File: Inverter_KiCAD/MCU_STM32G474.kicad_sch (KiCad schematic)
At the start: 27 parts, among them J2 Conn_ST_STDC14, SW1 SW_Push, SW2 SW_Push, SW3 SW_Push, SW4 SW_Push, U18 STM32G474RETx, Y1 16M

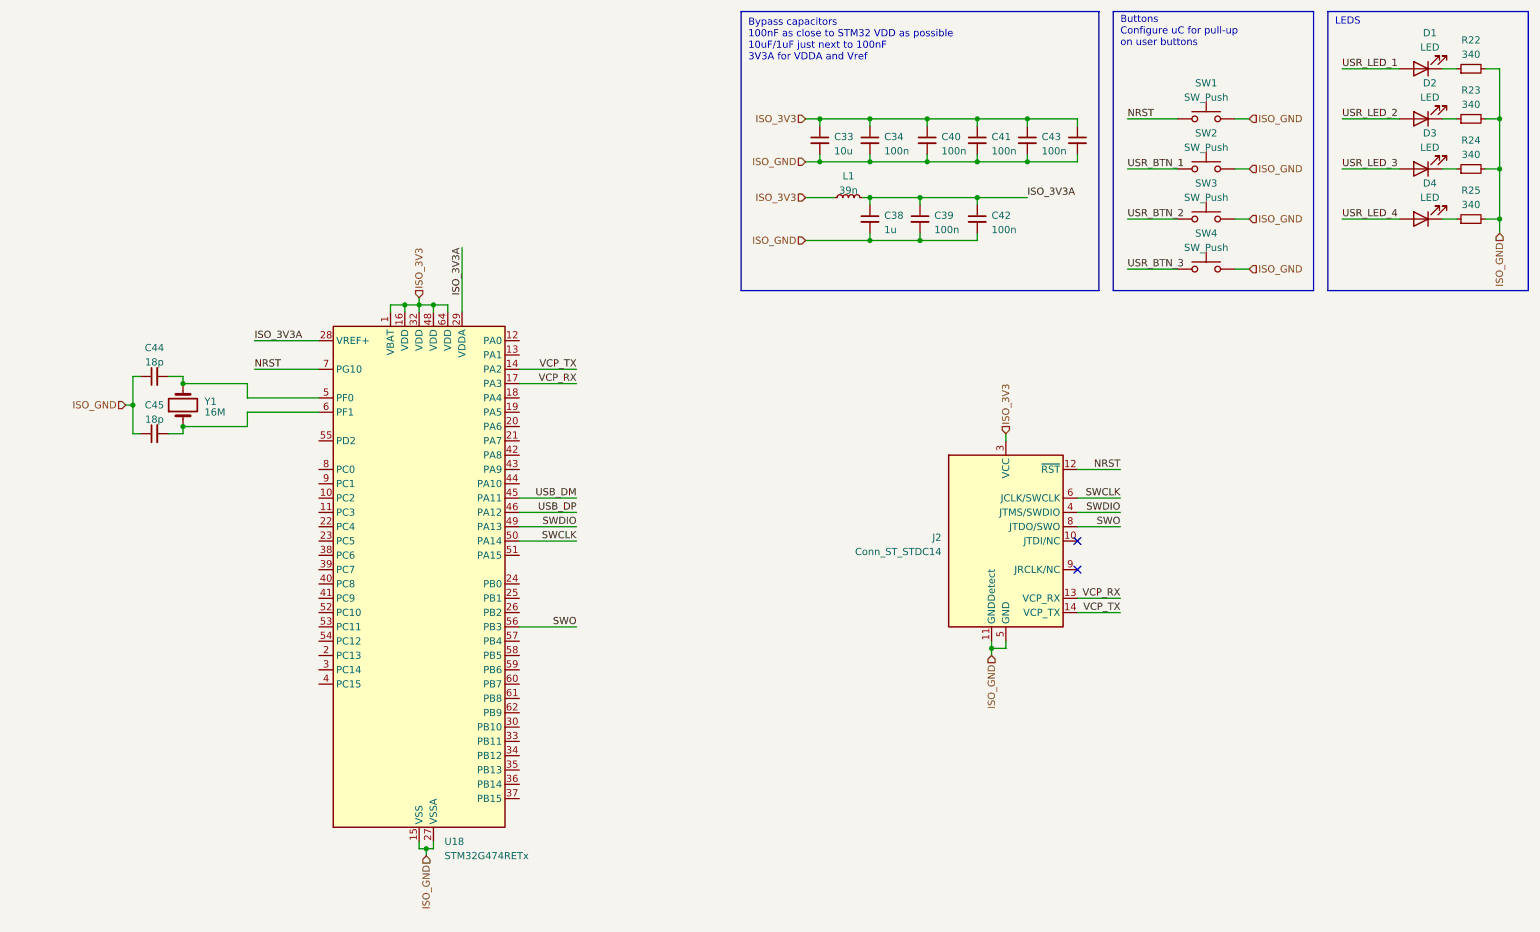
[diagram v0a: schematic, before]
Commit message: add break
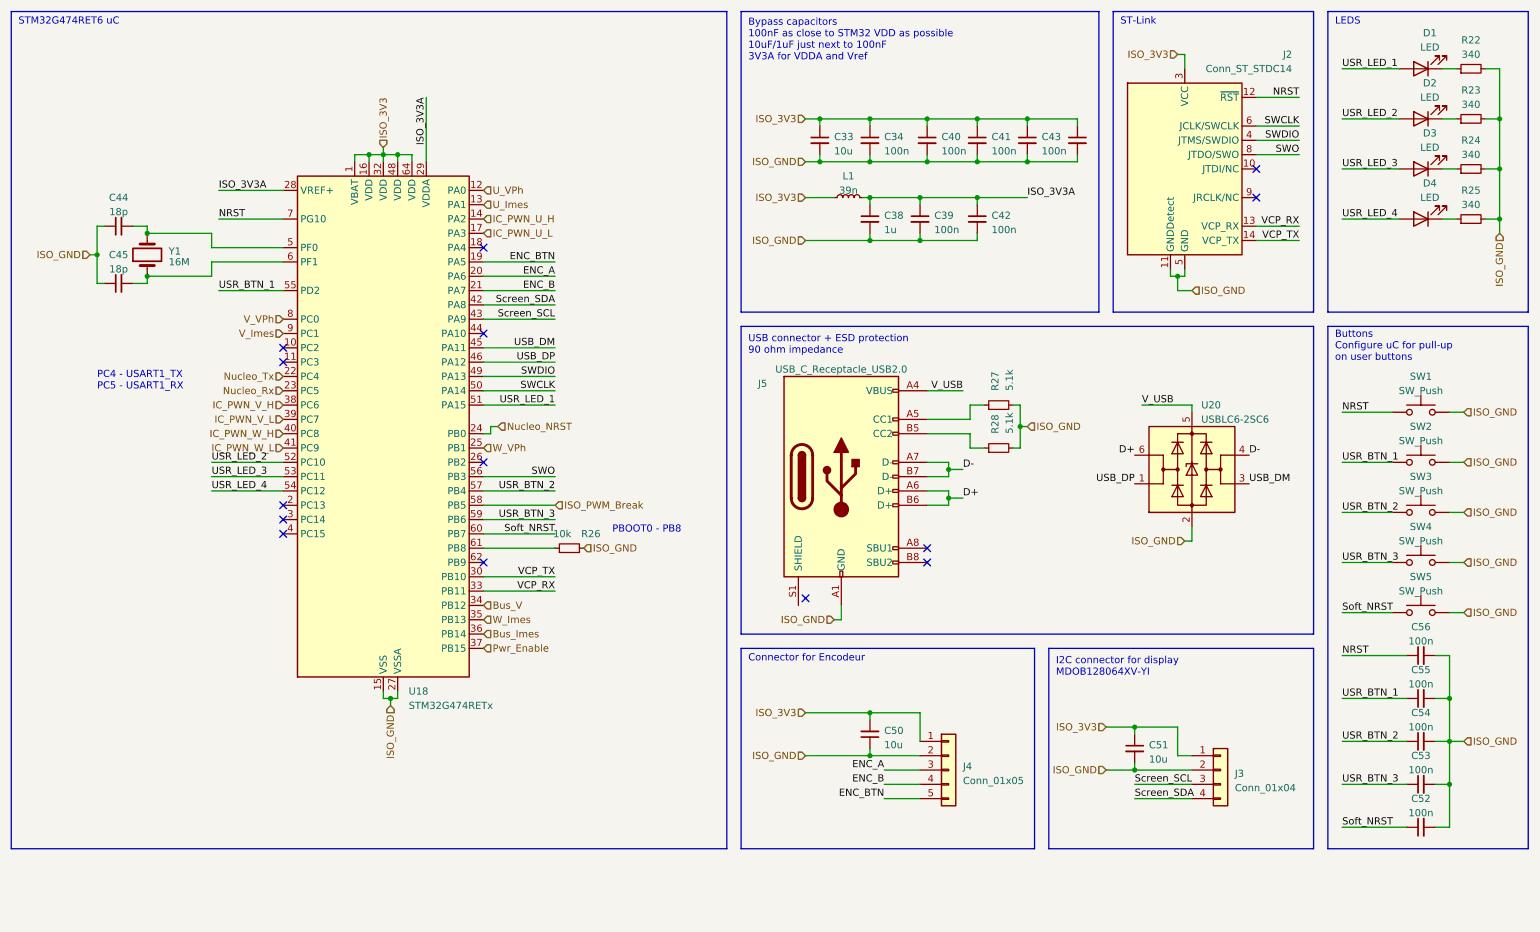
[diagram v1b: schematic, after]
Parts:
- added C50, C51: 10u, Capacitor_SMD:C_0603_1608Metric_Pad1.08x0.95mm_HandSolder, symbol Device:C_Small
- added C52, C53, C54, C55, C56: 100n, Capacitor_SMD:C_0402_1005Metric_Pad0.74x0.62mm_HandSolder, symbol Device:C_Small
- added J3: Conn_01x04, Connector_JST:JST_XH_B4B-XH-A_1x04_P2.50mm_Vertical, symbol Connector_Generic:Conn_01x04
- added J4: Conn_01x05, Connector_JST:JST_XH_B5B-XH-A_1x05_P2.50mm_Vertical, symbol Connector_Generic:Conn_01x05
- added J5: USB_C_Receptacle_USB2.0, Connector_USB:USB_C_Receptacle_HRO_TYPE-C-31-M-12, symbol Connector:USB_C_Receptacle_USB2.0
- added R26: 10k, Resistor_SMD:R_0603_1608Metric_Pad0.98x0.95mm_HandSolder, symbol Device:R_Small
- added R27, R28: 5.1k, Resistor_SMD:R_0603_1608Metric_Pad0.98x0.95mm_HandSolder, symbol Device:R_Small
- added SW5: SW_Push, Button_Switch_SMD:SW_SPST_B3U-3000P, symbol Switch:SW_Push
- added U20: USBLC6-2SC6, Package_TO_SOT_SMD:SOT-23-6, symbol Power_Protection:USBLC6-2SC6
- C33, C38: footprint (none) -> Capacitor_SMD:C_0603_1608Metric_Pad1.08x0.95mm_HandSolder
- C34, C39, C40, C41, C42, C43, C44, C45, C46: footprint (none) -> Capacitor_SMD:C_0402_1005Metric_Pad0.74x0.62mm_HandSolder
- D1, D2, D3, D4: footprint (none) -> LED_SMD:LED_0603_1608Metric_Pad1.05x0.95mm_HandSolder
- L1: footprint (none) -> Inductor_SMD:L_0603_1608Metric_Pad1.05x0.95mm_HandSolder
- R22, R23, R24, R25: footprint (none) -> Resistor_SMD:R_0603_1608Metric_Pad0.98x0.95mm_HandSolder
- SW1, SW2, SW3, SW4: footprint (none) -> Button_Switch_SMD:SW_SPST_B3U-3000P
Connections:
- net ISO_3V3: now also C50.2, C51.1, J3.1 (Pin_1), J4.1 (Pin_1)
- net ISO_GND: now also C50.1, C51.2, C52.2, C53.2, C54.2, C55.2, C56.2, J3.2 (Pin_2), J4.2 (Pin_2), J5.A1 (GND), J5.A12 (GND), J5.B1 (GND), J5.B12 (GND), R26.2, R27.2, R28.2, SW5.2, U20.2 (GND)
- net NRST: now also C56.1
- net USB_DM: now also U20.3 (I/O2)
- net USB_DP: now also U20.1 (I/O1)
- net USR_BTN_1: now also U18.55 (PD2), C55.1
- net USR_BTN_2: now also U18.57 (PB4), C54.1
- net USR_BTN_3: now also U18.59 (PB6), C53.1
- net USR_LED_1: now also U18.51 (PA15)
- net USR_LED_2: now also U18.52 (PC10)
- net USR_LED_3: now also U18.53 (PC11)
- net USR_LED_4: now also U18.54 (PC12)
- net VCP_RX: now also U18.33 (PB11); no longer U18.17 (PA3)
- net VCP_TX: now also U18.30 (PB10); no longer U18.14 (PA2)
- net U_VPh: now reaches U18.12 (PA0)
- net U_Imes: now reaches U18.13 (PA1)
- net ENC_BTN: now reaches U18.19 (PA5)
- net ENC_BTN: now also J4.5 (Pin_5)
- net ENC_A: now reaches U18.20 (PA6)
- net ENC_A: now also J4.3 (Pin_3)
- net ENC_B: now reaches U18.21 (PA7)
- net ENC_B: now also J4.4 (Pin_4)
- net Nucleo_Tx: now reaches U18.22 (PC4)
- net Nucleo_Rx: now reaches U18.23 (PC5)
- net Nucleo_NRST: now reaches U18.24 (PB0)
- net W_VPh: now reaches U18.25 (PB1)
- net Bus_V: now reaches U18.34 (PB12)
- net W_Imes: now reaches U18.35 (PB13)
- net Bus_Imes: now reaches U18.36 (PB14)
- net Pwr_Enable: now reaches U18.37 (PB15)
- net IC_PWN_V_H: now reaches U18.38 (PC6)
- net IC_PWN_V_L: now reaches U18.39 (PC7)
- net IC_PWN_W_H: now reaches U18.40 (PC8)
- net IC_PWN_W_L: now reaches U18.41 (PC9)
- net Screen_SDA: now reaches U18.42 (PA8)
- net Screen_SDA: now also J3.4 (Pin_4)
- net Screen_SCL: now reaches U18.43 (PA9)
- net Screen_SCL: now also J3.3 (Pin_3)
- net ISO_PWM_Break: now reaches U18.58 (PB5)
- net Soft_NRST: now reaches U18.60 (PB7)
- net Soft_NRST: now also C52.1, SW5.1
- net at U18.61 (PB8): now also R26.1
- net V_VPh: now reaches U18.8 (PC0)
- net V_Imes: now reaches U18.9 (PC1)
- new net: J5.B5 (CC2), R28.1
- new net: J5.A5 (CC1), R27.1
- new net D+: J5.A6 (D+), J5.B6 (D+), U20.6 (I/O1)
- new net D-: J5.A7 (D-), J5.B7 (D-), U20.4 (I/O2)
- new net IC_PWN_U_H: U18.14 (PA2)
- new net IC_PWN_U_L: U18.17 (PA3)
- new net V_USB: J5.A4 (VBUS), J5.A9 (VBUS), J5.B4 (VBUS), J5.B9 (VBUS), U20.5 (VBUS)
- no-connect marks 2 -> 14
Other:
- note added: "Connector for Encodeur"
- note added: "I2C connector for display MDOB128064XV-YI"
- note added: "PBOOT0 - PB8"
- note added: "PC4 - USART1_TX PC5 - USART1_RX"
- note added: "ST-Link"
- note added: "STM32G474RET6 uC"
- note added: "USB connector + ESD protection 90 ohm impedance"
- moved on the sheet: C44, C45, J2, SW1, SW2, SW3, SW4, U18, Y1
